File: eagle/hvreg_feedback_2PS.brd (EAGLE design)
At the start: 119.6 x 108.5 mm, 37 parts, among them K1 G5V-2, X4 BU-SMA-V

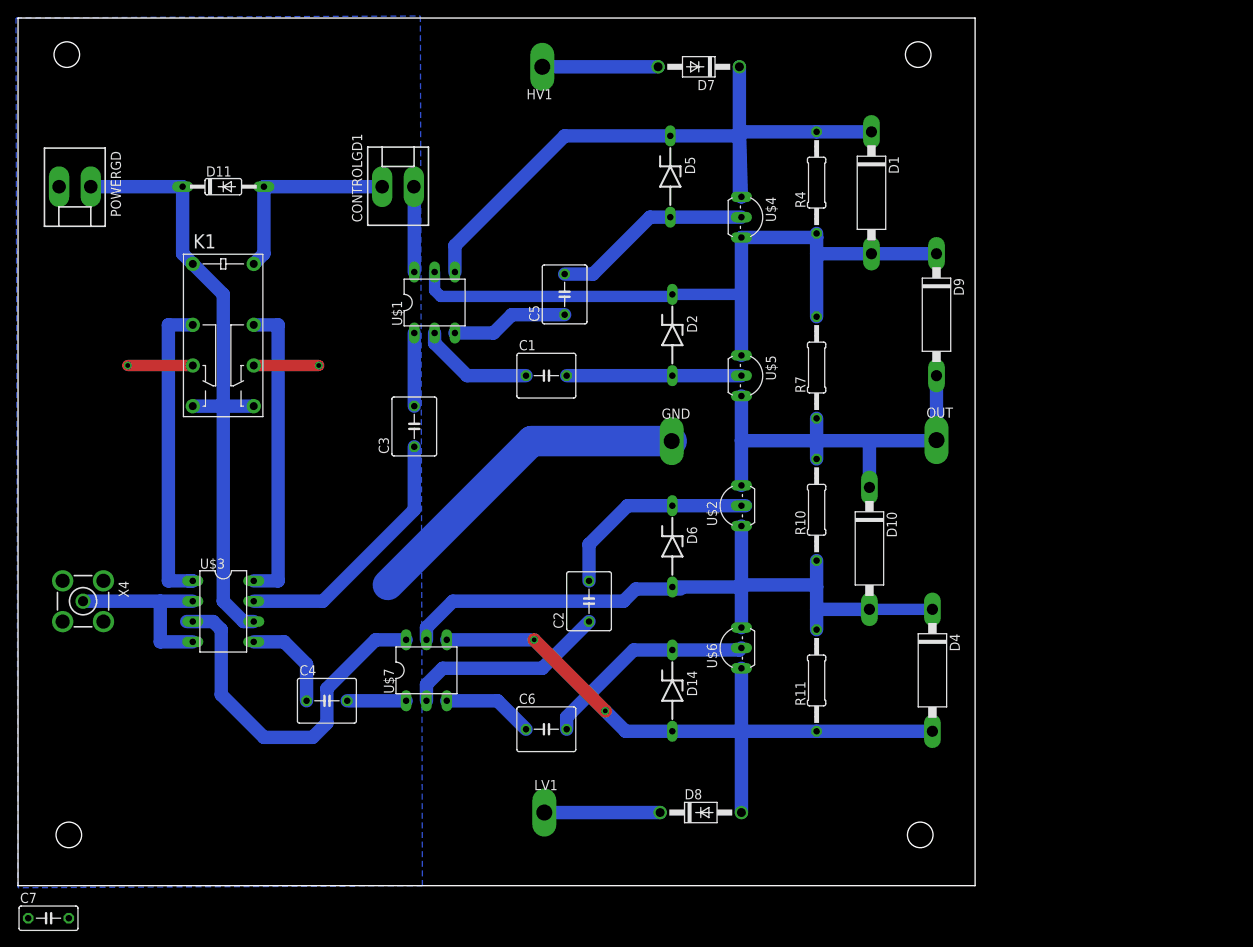
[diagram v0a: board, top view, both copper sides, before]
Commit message: feedback on hv rails
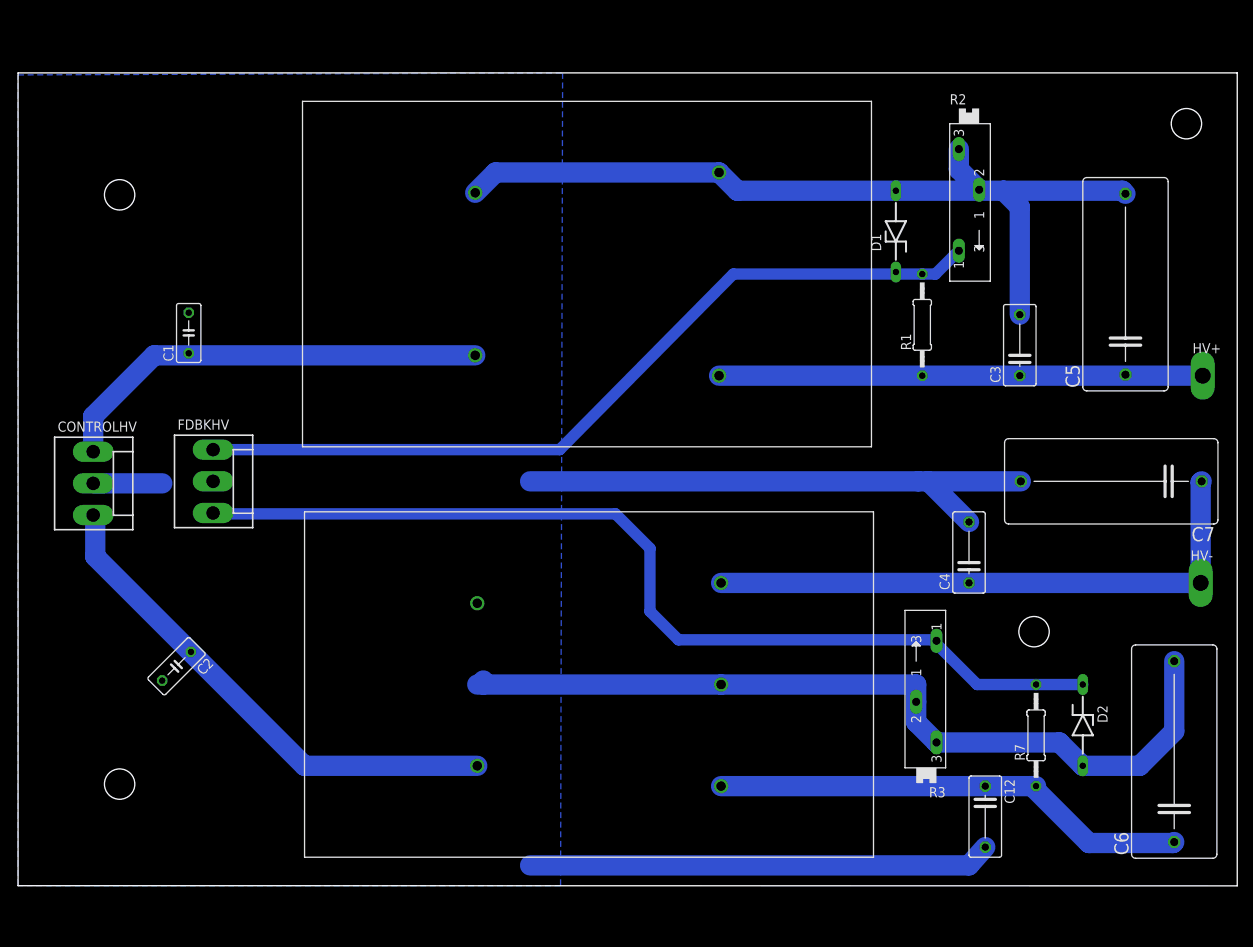
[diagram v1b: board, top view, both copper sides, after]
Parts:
- removed CONTROLGD1, POWERGD: (no value), con-molex:KK-156-2
- removed D10, D4, D9: P6KEXXA, diode:C1702-15
- removed D11: 1N4148DO35-10, diode:DO35-10
- removed D14, D5, D6: 4742, diode:ZDIO-10
- removed D7, D8: 1N4004, diode:DO41-10
- removed GND, HV1, LV1, OUT: TPPAD1-20Y, testpad:P1-20Y
- removed K1: G5V-2, relay:G5V-2
- removed R10, R11, R4: 1M, rcl:0207/12
- removed U$3: UCC27425, texas:DIL08
- removed U$4, U$5: VP0550, transistor-fet:TO92-
- removed U$6: VN0550, transistor-fet:TO92-
- removed U$7: DA-2320, trafo:DIL06
- removed X4: BU-SMA-V, con-coax:BU-SMA-V
- added C12: .01u, rcl:C075-042X103
- added CONTROLHV, FDBKHV: (no value), con-molex:KK-156-3
- added HV+, HV-: TPPAD1-20Y, testpad:P1-20Y
- added R1: 2M, resistor:0207/12
- added R2, R3: (no value), pot:SP19L
- C1, C2: device resistor:C050-055X075 -> rcl:C050-030X075
- C3, C4: value (none) -> .01u; device resistor:C050-055X075 -> rcl:C075-042X103
- C5, C6: value (none) -> 1u; device resistor:C050-055X075 -> rcl:C225-108X268
- C7: value (none) -> 1u; device rcl:C050-030X075 -> rcl:C225-108X268
- D1: value P6KEXXA -> 1n4733; device diode:C1702-15 -> diode:ZDIO-10
- D2: value 4742 -> 1n4733
- R7: value 1M -> 2M; device rcl:0207/12 -> resistor:0207/12
- U$1: value DA-2320 -> EMCO-F104PIN; device trafo:DIL06 -> dc-dc-converter:EMCO-F
- U$2: value VN0550 -> EMCO-F20CT; device transistor-fet:TO92- -> dc-dc-converter:EMCO-F*CT
- moved C7 143.6 mm to (136.7, 50.5), turned to 180 degrees
- moved C4 82.4 mm to (118.9, 41.7), turned to 90 degrees
- moved C6 78.5 mm to (144.5, 16.8), turned to 90 degrees
- moved C3 76.4 mm to (125.2, 67.6)
- moved D2 70.8 mm to (133.1, 20.1)
- moved C5 70.1 mm to (138.4, 75.2)
- moved R7 53.5 mm to (127.3, 18.8)
- moved C2 52.2 mm to (19.8, 27.4), turned to 225 degrees
- moved U$2 46.3 mm to (57.4, 15.0), turned to 0 degrees
- moved C1 45.0 mm to (21.3, 69.1), turned to 90 degrees
- moved U$1 8.33 mm to (57.1, 66.3)
- moved D1 5.71 mm to (109.7, 81.8), turned to 90 degrees
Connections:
- removed net +15V: C7.1, D11.C, K1.1, K1.8, K1.9, POWERGD.1, U$3.6
- removed net ENSW: CONTROLGD1.1, D11.A, K1.16
- removed net N$10: D8.C, LV1.TP
- removed net N$11: C1.2, D2.A, U$5.2
- removed net N$13: D10.A, D4.C, D6.A, R10.1, R11.2, U$2.3, U$6.1
- removed net N$14: K1.4, U$3.1
- removed net N$15: K1.13, U$3.8
- removed net N$16: C5.2, D5.A, U$4.2
- removed net N$17: D1.C, D5.C, D7.C, R4.2, U$1.4, U$4.3
- removed net N$18: D1.A, D2.C, D9.C, R4.1, R7.2, U$1.5, U$4.1, U$5.3
- removed net N$21: D10.C, D9.A, OUT.TP, R10.2, R7.1, U$2.1, U$5.1
- removed net N$22: C2.1, U$7.2
- removed net N$23: C6.1, U$7.3
- removed net N$25: C2.2, D6.C, U$2.2
- removed net N$27: C6.2, D14.C, U$6.2
- removed net N$29: D7.A, HV1.TP
- removed net N$30: D14.A, D4.A, D8.A, R11.1, U$6.3, U$7.4
- removed net N$7: C5.1, U$1.3
- removed net N$9: U$7.5
- new net N$8: D2.C, FDBKHV.3, R3.A, R7.2
- net GND: now also C1.2, C12.2, C2.2, C3.2, C4.2, C5.2, C6.2, CONTROLHV.2, D1.A, D2.A, FDBKHV.2, R2.E, R2.S, R3.E, R3.S, U$1.P$2, U$1.P$4, U$2.P$2, U$2.P$5; no longer CONTROLGD1.2, GND.TP, K1.11, K1.6, POWERGD.2, U$1.6, U$3.3, U$7.6, X4.2, X4.3, X4.4, X4.5
- net N$1: now also C3.1, C5.1, HV+.TP, R1.1, U$1.P$3; no longer U$3.2, U$3.4, X4.1
- net N$2: now also C12.1, C6.1, R7.1, U$2.P$3; no longer C3.1, U$3.7
- net N$3: now also D1.C, FDBKHV.1, R1.2, R2.A; no longer C3.2, U$1.1
- net N$4: now also C1.1, CONTROLHV.1, U$1.P$1; no longer C4.1, U$3.5
- net N$5: now also C2.1, CONTROLHV.3, U$2.P$1; no longer C1.1, U$1.2
- net N$6: now also C4.1, C7.1, HV-.TP, U$2.P$4; no longer C4.2, U$7.1
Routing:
- net GND: track 115.7 -> 346.1 mm, vias 2 -> 0
- net N$8: track 0.00 -> 122.2 mm
- net N$3: track 9.14 -> 103.6 mm
- net N$18: track 90.7 -> 0.00 mm
- net N$17: track 85.6 -> 0.00 mm
- net N$30: track 83.5 -> 0.00 mm, vias 2 -> 0
- net +15V: track 77.9 -> 0.00 mm
- net N$6: track 7.37 -> 72.7 mm
- net N$13: track 55.6 -> 0.00 mm
- net N$21: track 54.6 -> 0.00 mm
- net N$5: track 14.4 -> 63.9 mm
- net N$4: track 12.3 -> 55.3 mm
- net N$14: track 38.6 -> 0.00 mm
- net N$15: track 38.1 -> 0.00 mm
- net N$1: track 22.9 -> 60.5 mm
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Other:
- board size 119.6 x 108.5 mm -> 152.4 x 101.6 mm
